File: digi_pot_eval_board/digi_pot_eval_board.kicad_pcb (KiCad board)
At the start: 2 copper layers, 103.6 x 162.6 mm, 82 parts, among them J1 Conn_01x07_Male, J10 AudioJack3, J11 Conn_01x02_Male, J12 Conn_01x03_Male, J13 Conn_01x06_Male, J2 Conn_01x10_Male, J3 47346-0001, J4 DS-210, J5 DIN-5-OOTDTY, J6 DIN-5-OOTDTY, J7 JST-04, J8 DS1013-06S, J9 AudioJack3, K2 G6K2FYTR5DC, K4 G6K2FYTR5DC, K5 G6K2FYTR5DC, K6 G6K2FYTR5DC, K7 G6K2FYTR5DC, Q1 BSS84, Q2 BSS84, SW3 SW_Push, U1 DigiPot, U10 6N138, U11 NCP1117ST50T3G, U12 ATmega32U4-AU, U2 DigiPot, U3 DigiPot, U4 DigiPot, U5 DigiPot, U6 DigiPot, U7 DigiPot, U8 ULN2003A, U9 USBLC6-2SC6, Y1 16MHz HC-49SM

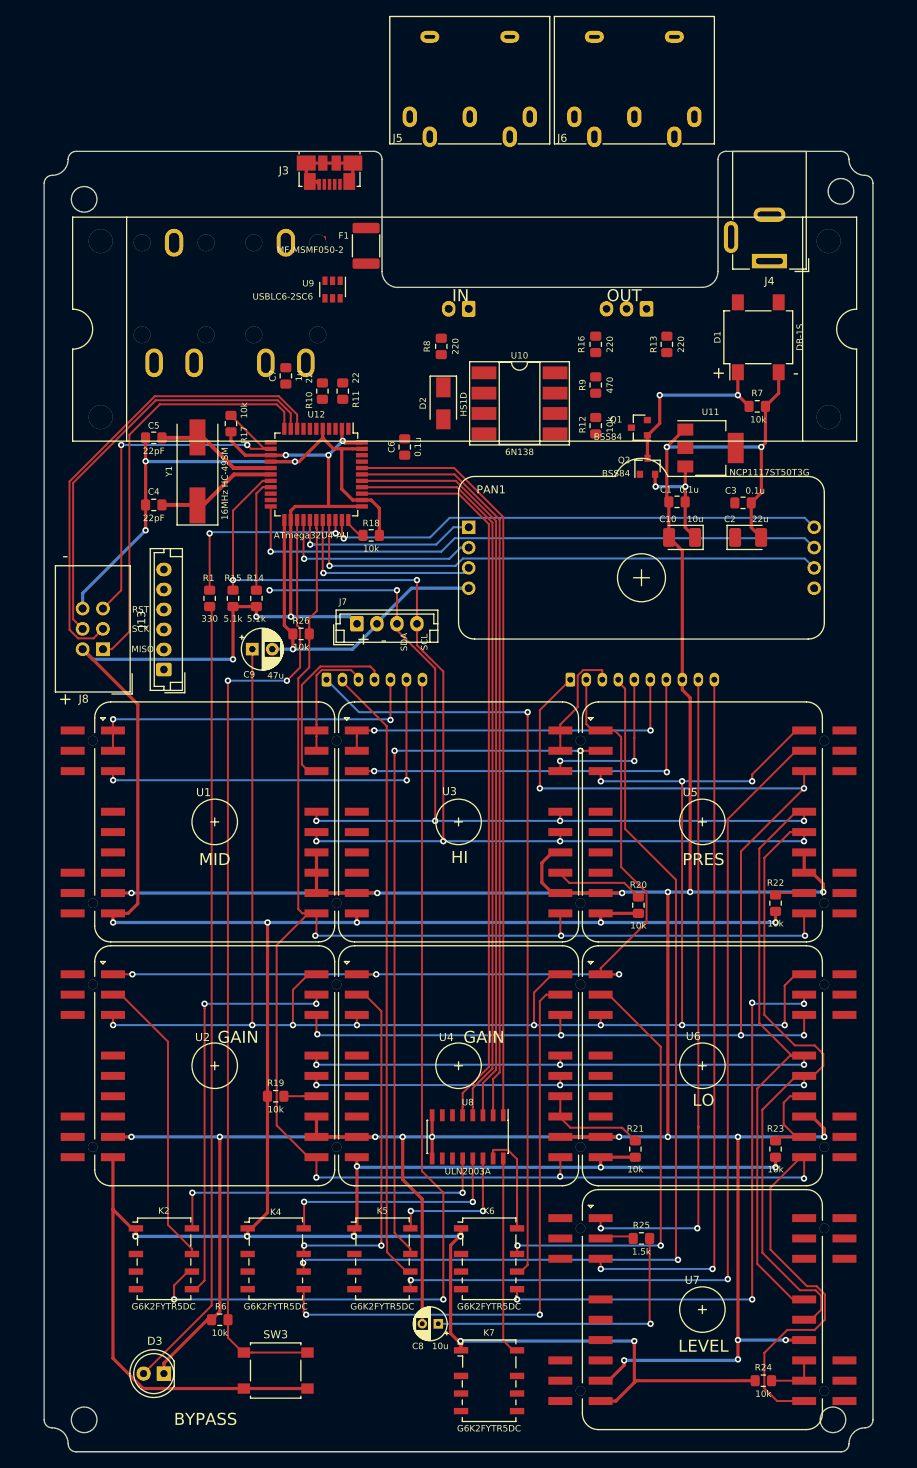
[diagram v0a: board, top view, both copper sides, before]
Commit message: Introducing new layout.
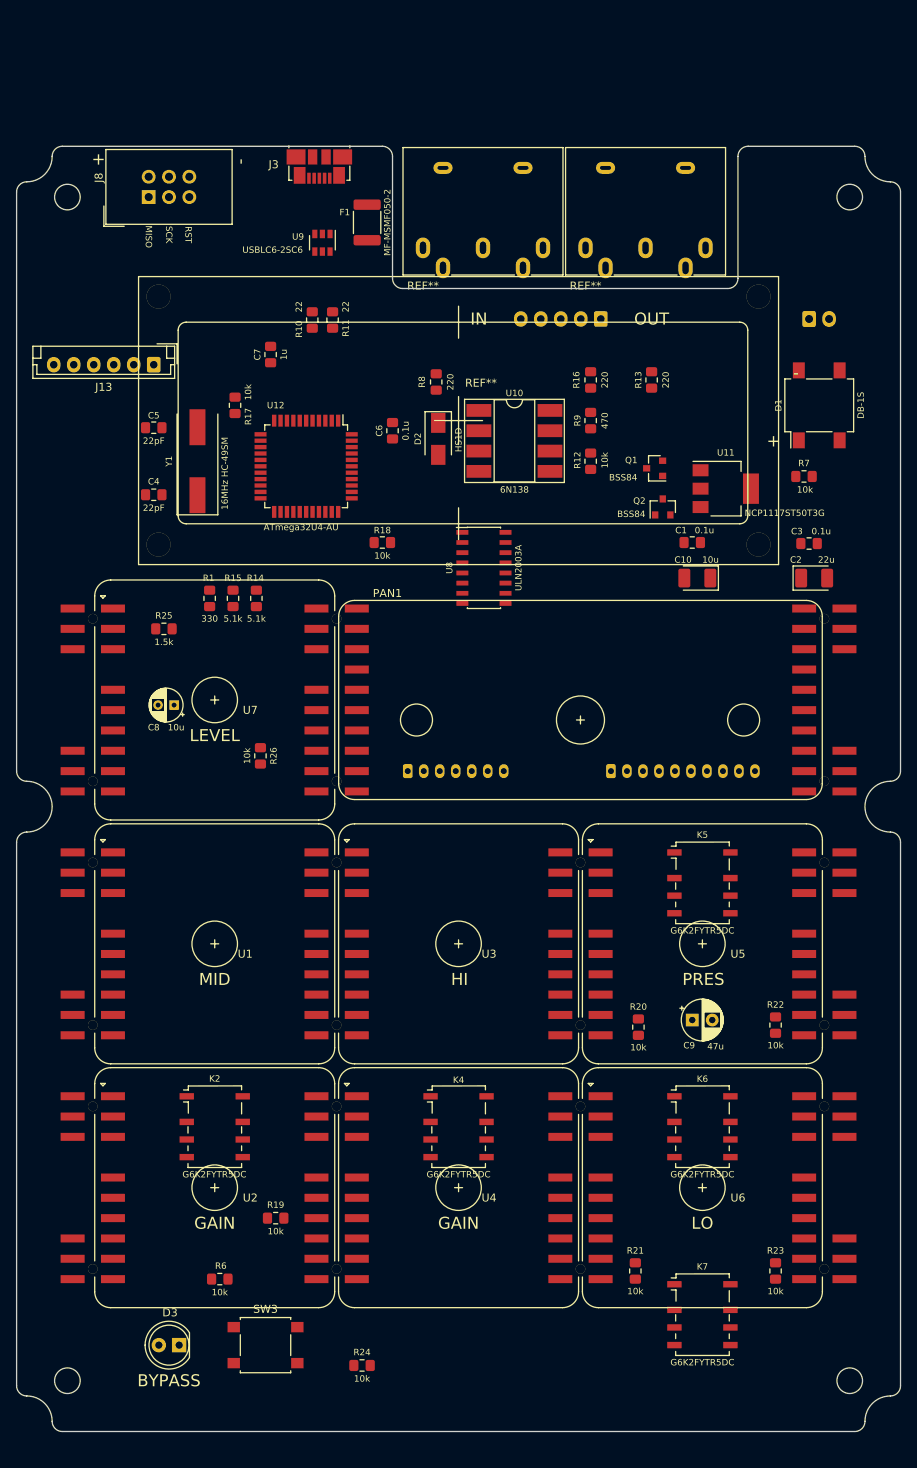
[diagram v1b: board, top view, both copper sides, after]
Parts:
- removed J11: Conn_01x02_Male, Connector_JST:JST_EH_B02B-EH-A_1x02_P2.50mm_Vertical
- removed J12: Conn_01x03_Male, Connector_JST:JST_EH_B03B-EH-A_1x03_P2.50mm_Vertical
- removed J4: DS-210, Connector_BarrelJack:BarrelJack_Wuerth_6941xx301002
- removed J5, J6: DIN-5-OOTDTY, Connectors:DIN5MIDI-OOTDTY
- removed J7: JST-04, Connector_JST:JST_EH_B04B-EH-A_1x04_P2.50mm_Vertical
- removed the REF** at (163.4, 34.2)
- removed the REF** at (116.3, 51.4)
- removed the REF** at (68.8, 35.2)
- added REF**: DIN-5-OOTDTY, Connectors:DIN5MIDI-OOTDTY, F.Cu at (131.4, 41.3)
- added REF**: DISPLAY, OLED:oled1602, F.Cu at (115.6, 62.9)
- added REF**: MountingHole_3.2mm_M3_DIN965, MountingHole:MountingHole_3.2mm_M3_DIN965, F.Cu at (164.5, 34.9)
- added REF**: MountingHole_3.2mm_M3_DIN965, MountingHole:MountingHole_3.2mm_M3_DIN965, F.Cu at (66.7, 34.9)
- added REF**: DIN-5-OOTDTY, Connectors:DIN5MIDI-OOTDTY, F.Cu at (111.1, 41.3)
- J10: value AudioJack3 -> Conn_01x02_Male; footprint Connectors:phone-jack-6.3 -> Connector_JST:JST_EH_B02B-EH-A_1x02_P2.50mm_Vertical
- J9: value AudioJack3 -> Conn_01x05_Male; footprint Connectors:phone-jack-6.3 -> Connector_JST:JST_EH_B05B-EH-A_1x05_P2.50mm_Vertical
- PAN1: footprint nav_panel:nav_panel_THT -> nav_panel:nav_panel_SMD
- moved U7 97.6 mm to (71.1, 86.4)
- moved ? 97.6 mm to (68.6, 109.2)
- moved R25 96.8 mm to (78.7, 88.9)
- moved C8 84.1 mm to (80.0, 98.4)
- moved J10 79.9 mm to (159.4, 50.2), turned to 0 degrees
- moved ? 76.2 mm to (162.6, 86.4)
- moved C9 71.9 mm to (144.8, 137.8)
- moved U8 71.1 mm to (118.7, 81.3), turned to 0 degrees
- moved K5 61.7 mm to (146.1, 120.7)
- moved J8 56.8 mm to (76.8, 34.9), turned to 90 degrees
- moved R24 50.2 mm to (103.5, 181.0)
- moved J9 40.5 mm to (133.3, 50.2), turned to 180 degrees
- moved J13 38.1 mm to (77.5, 55.9), turned to 180 degrees
- moved K6 31.4 mm to (146.1, 151.1)
- moved K4 28.2 mm to (115.6, 151.1)
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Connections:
- D1 pad 3: Net-(D1-Pad3) -> POW2
- D1 pad 4: Net-(D1-Pad4) -> POW1
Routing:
- net GND: track 604.9 -> 0.00 mm, vias 25 -> 0
- net +5V: track 495.4 -> 0.00 mm, vias 20 -> 0
- net SCL: track 281.9 -> 0.00 mm, vias 9 -> 0
- net CHG: track 271.6 -> 0.00 mm, vias 6 -> 0
- net SDA: track 263.6 -> 0.00 mm, vias 9 -> 0
- net C: track 220.5 -> 0.00 mm, vias 11 -> 0
- net A3: track 153.0 -> 0.00 mm, vias 6 -> 0
- net HW: track 123.8 -> 0.00 mm, vias 2 -> 0
- net SW_PASSBACK: track 121.1 -> 0.00 mm, vias 2 -> 0
- net MW: track 117.0 -> 0.00 mm, vias 2 -> 0
- net A1: track 111.9 -> 0.00 mm, vias 3 -> 0
- net PW1: track 111.4 -> 0.00 mm, vias 2 -> 0
- net Net-(D3-Pad2): track 99.5 -> 0.00 mm
- net LW: track 97.6 -> 0.00 mm, vias 1 -> 0
- net KBP: track 95.0 -> 0.00 mm
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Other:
- board size 103.6 x 162.6 mm -> 110.5 x 160.7 mm
- board text removed: "SCL"
- board text removed: "SDA"
